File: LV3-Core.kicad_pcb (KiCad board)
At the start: 2 copper layers, 114.3 x 59.1 mm, 81 parts, among them IC1 TLV74033PDBVR, J1 Conn_01x02_Pin, J2 USB_C_Receptacle_USB2.0_16P, J3 Conn_01x01, J4 Conn_01x40_Socket, J5 Conn_01x05_Pin, J6 Conn_01x05_Pin, J7 Conn_01x01, J8 FTSH-105-01-L-DV-K-A, J9 Conn_01x02_Pin, U1 STM32G474RCTx, U2 TJA1051T-3, U3 TJA1051T-3, U4 LMR51625YDDCR, Y1 Crystal_GND24

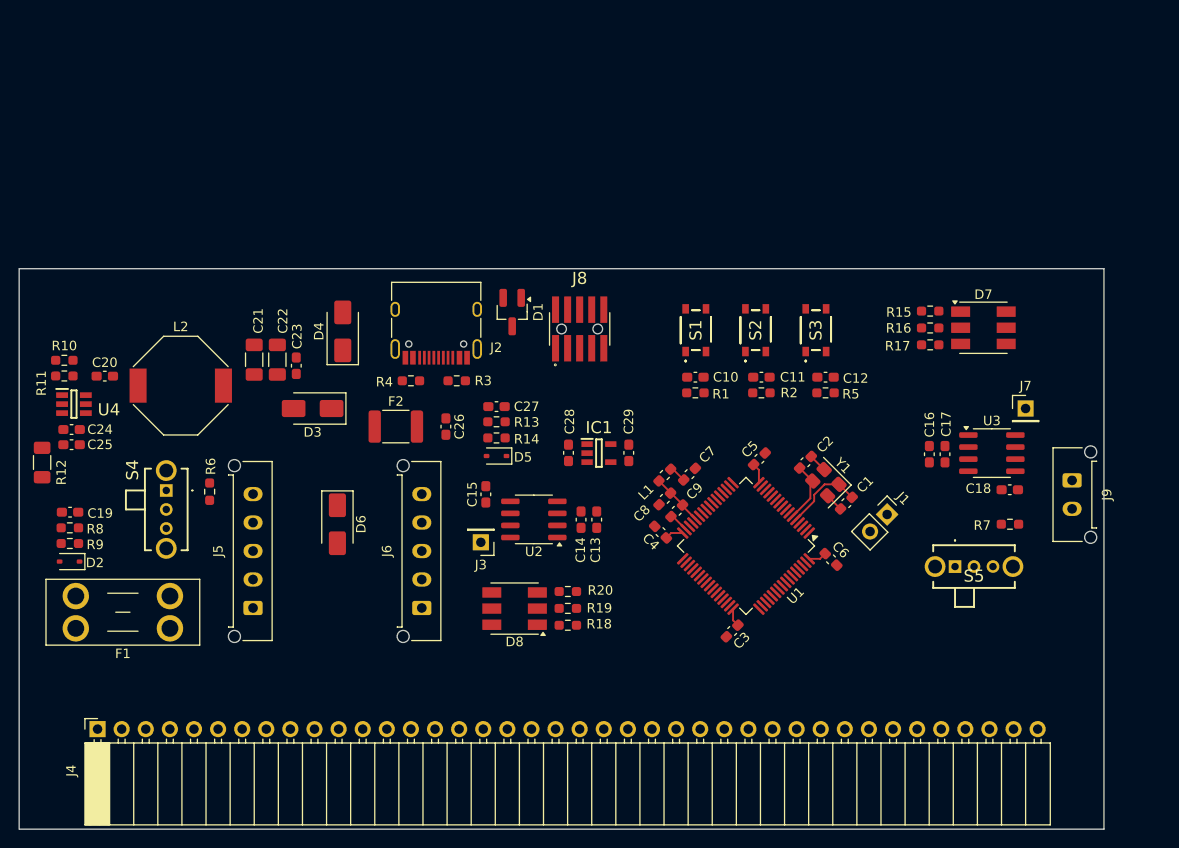
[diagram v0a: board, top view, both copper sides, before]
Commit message: layout almost complete
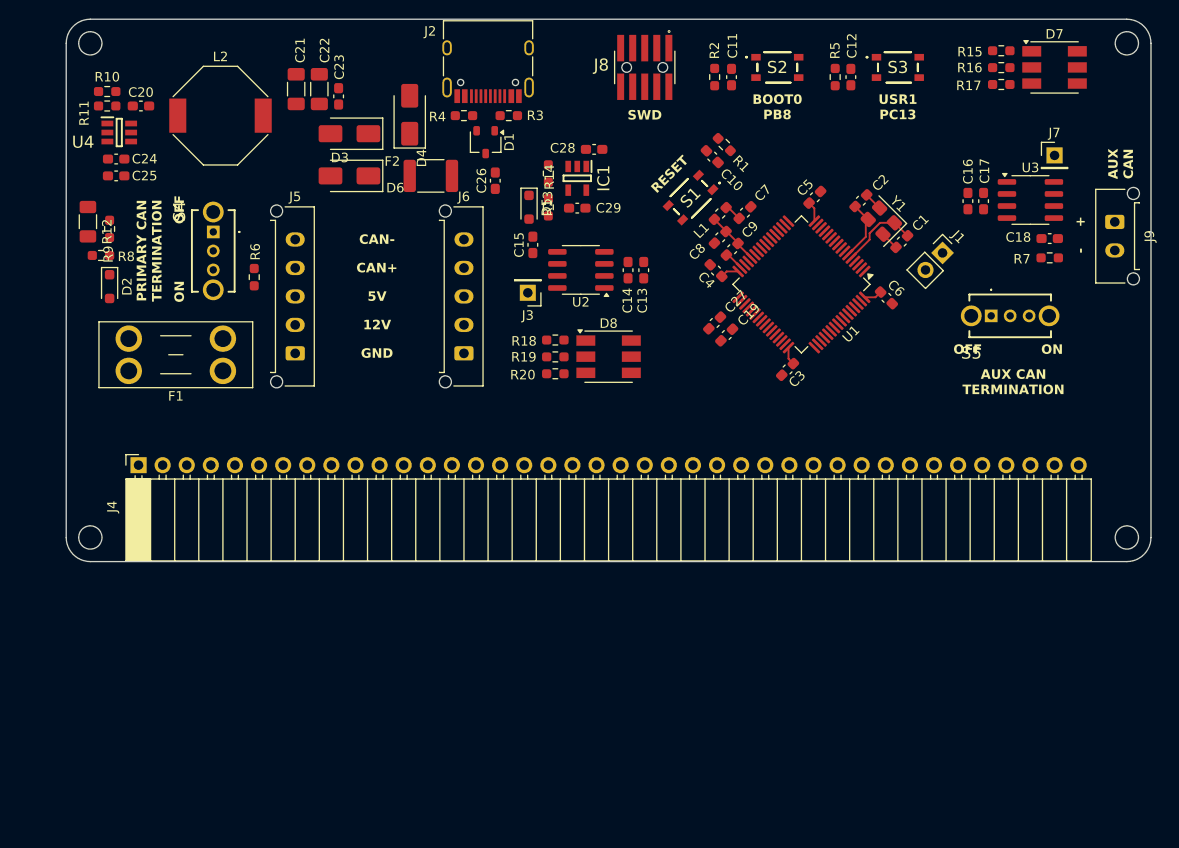
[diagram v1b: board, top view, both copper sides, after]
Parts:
- D1: footprint Package_TO_SOT_SMD:SOT-23_Handsoldering -> Package_TO_SOT_SMD:SOT-23W
- D2, D5: footprint Diode_SMD:D_SOD-323 -> Diode_SMD:D_SOD-323_HandSoldering
- moved C19 71.7 mm to (164.8, 96.8), turned to -135 degrees
- moved D6 36.7 mm to (125.1, 80.0), turned to 180 degrees
- moved R2 33.6 mm to (163.6, 69.6), turned to 90 degrees
- moved R9 33.4 mm to (99.8, 85.6), turned to 90 degrees
- moved R5 33.3 mm to (176.3, 69.6), turned to 90 degrees
- moved C28 32.1 mm to (150.9, 77.2), turned to 0 degrees
- moved C11 31.8 mm to (165.4, 69.6), turned to -90 degrees
- moved C12 31.7 mm to (177.9, 69.6), turned to -90 degrees
- moved R18 30.1 mm to (146.8, 97.3), turned to 0 degrees
- moved D2 29.3 mm to (99.8, 91.7), turned to -90 degrees
- moved D3 29.2 mm to (125.1, 75.6)
- moved IC1 29.0 mm to (149.1, 80.3), turned to -90 degrees
- moved U4 29.0 mm to (100.8, 75.4)
- moved S3 29.0 mm to (182.9, 68.6), turned to 0 degrees
- moved R8 28.9 mm to (98.9, 88.4)
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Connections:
- R6 pad 1: PRIMARY_CAN- -> PRIMARY_CAN+
- R7 pad 1: AUX_CAN- -> AUX_CAN+
- S4 pad 2: PRIMARY_CAN+ -> PRIMARY_CAN-
- S5 pad 2: AUX_CAN+ -> AUX_CAN-
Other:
- board size 114.3 x 59.1 mm -> 114.3 x 57.2 mm
- board text added: "+"
- board text added: "-"
- board text added: "12V"
- board text added: "5V"
- board text added: "AUX CAN"
- board text added: "AUX CAN TERMINATION"
- board text added: "BOOT0 PB8"
- board text added: "CAN+"
- board text added: "CAN-"
- board text added: "GND"
- board text added: "OFF"
- board text added: "ON"
- board text added: "PRIMARY CAN TERMINATION"
- board text added: "RESET"
- board text added: "SWD"
- board text added: "USR1 PC13"
